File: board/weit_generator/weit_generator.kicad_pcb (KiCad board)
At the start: 2 copper layers, 46 parts, among them J1 POWER, J2 PROG, J3 OUTPUT, U1 MCP6004, U2 AVR32DA28x-xSO, U3 TL431DBZ, X1 SG-5032CCN

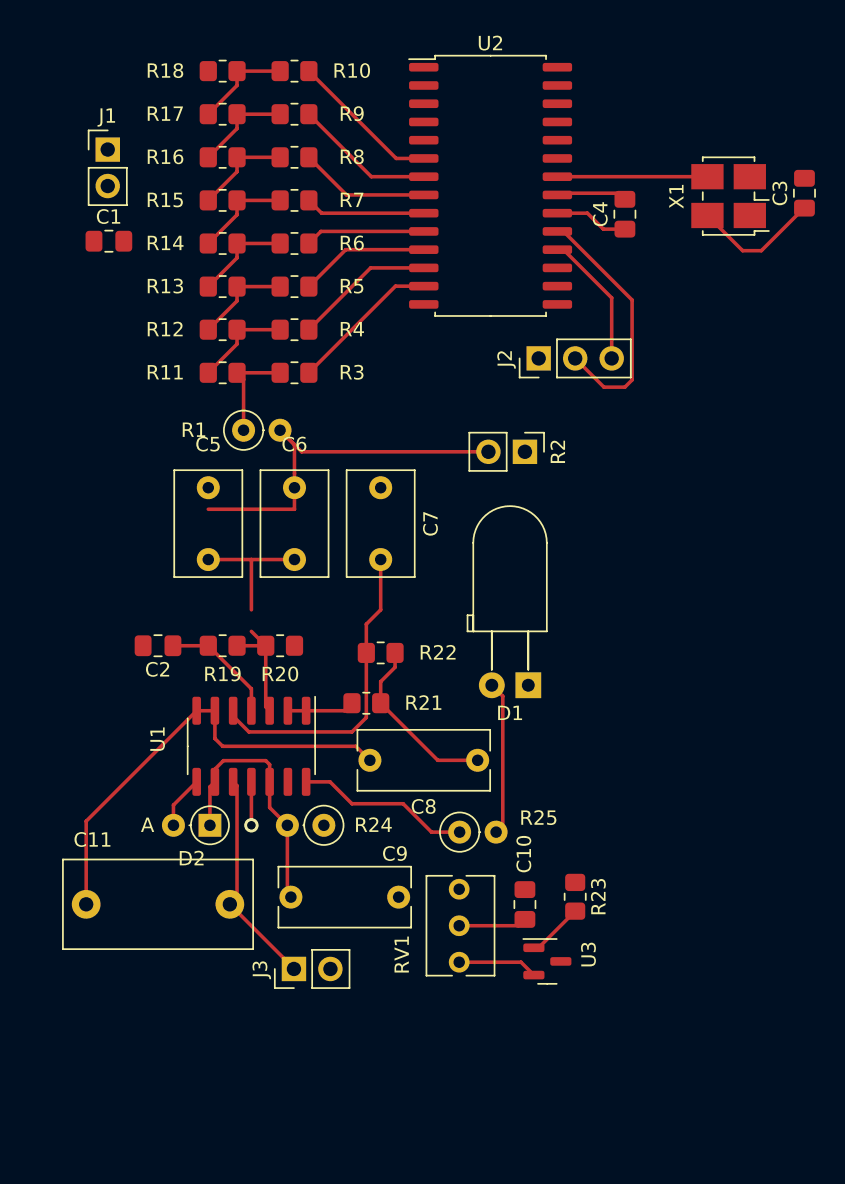
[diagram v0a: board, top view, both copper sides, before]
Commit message: .
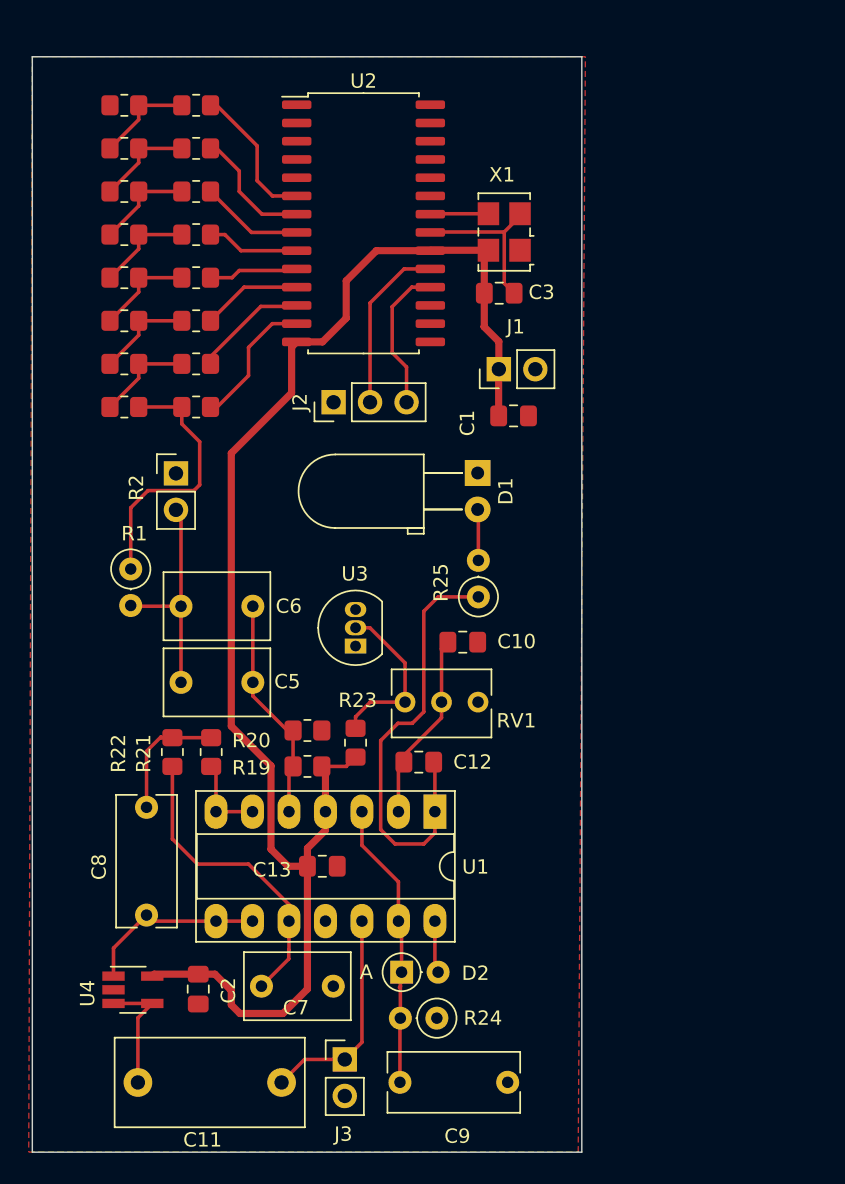
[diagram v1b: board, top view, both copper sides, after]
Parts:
- removed C4: 100n, Capacitor_SMD:C_0805_2012Metric_Pad1.18x1.45mm_HandSolder
- added C12: 1n, Capacitor_SMD:C_0805_2012Metric_Pad1.18x1.45mm_HandSolder, F.Cu at (159.7, 114.1)
- added C13: 100n, Capacitor_SMD:C_0805_2012Metric_Pad1.18x1.45mm_HandSolder, F.Cu at (152.9, 121.3)
- added U4: LMV321, Package_TO_SOT_SMD:SOT-23-5_HandSoldering, F.Cu at (139.8, 129.9)
- R25: value 50 -> 1k
- U1: footprint Package_SO:SOIC-14_3.9x8.7mm_P1.27mm -> Package_DIP:DIP-14_W7.62mm_Socket_LongPads
- U3: value TL431DBZ -> LM4041LP-ADJ; footprint Package_TO_SOT_SMD:SOT-23 -> Package_TO_SOT_THT:TO-92_Inline
- X1: value SG-5032CCN -> SG-5032CAN; footprint Oscillator:Oscillator_SMD_SeikoEpson_SG8002LB-4Pin_5.0x3.2mm_HandSoldering -> Oscillator:Oscillator_SMD_SeikoEpson_SG8002LB-4Pin_5.0x3.2mm
- moved C7 34.9 mm to (153.7, 129.7), turned to 180 degrees
- moved J1 31.2 mm to (165.2, 86.8), turned to 90 degrees
- moved C1 30.7 mm to (166.2, 90.0)
- moved U3 25.7 mm to (155.2, 106.0), turned to 90 degrees
- moved R2 24.3 mm to (142.8, 94.0), turned to 0 degrees
- moved C2 24.1 mm to (144.3, 129.9), turned to -90 degrees
- moved C8 23.3 mm to (140.7, 117.2), turned to -90 degrees
- moved C3 22.4 mm to (165.2, 81.5), turned to 0 degrees
- moved C10 18.8 mm to (162.7, 105.8), turned to 0 degrees
- moved R23 18.7 mm to (155.2, 112.8), turned to 90 degrees
- moved D2 16.8 mm to (158.5, 128.7), turned to 0 degrees
- moved R25 16.4 mm to (163.8, 102.6), turned to 90 degrees
- moved R22 16.1 mm to (142.5, 113.4), turned to -90 degrees
- moved X1 15.8 mm to (165.6, 77.2)
- moved R24 15.6 mm to (160.9, 131.9)
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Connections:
- C10 pad 1: Net-(U1D--) -> Net-(U1A--)
- C11 pad 1: /Output Filter/OUT -> Net-(U4--)
- C5 pad 1: Net-(U1A-+) -> Net-(U1B-+)
- C6 pad 1: Net-(U1A-+) -> Net-(U1B-+)
- C7 pad 2: Net-(U1B-+) -> Net-(U1C-+)
- R19 pad 2: Net-(U1A-+) -> Net-(U1B-+)
- R20 pad 2: Net-(U1A-+) -> Net-(U1B-+)
- R21 pad 1: Net-(U1A--) -> Net-(U1B--)
- R22 pad 2: Net-(U1B-+) -> Net-(U1C-+)
- R25 pad 1: Net-(R25-Pad1) -> Net-(C12-Pad1)
- RV1 pad 2: Net-(U1D--) -> Net-(U1A--)
- U1 pad 1: Net-(U1A--) -> Net-(C12-Pad1)
- U1 pad 10: /OUTPUT -> Net-(U1C-+)
- U1 pad 12: Net-(D2-K) -> /OUTPUT
- U1 pad 13: Net-(U1D--) -> Net-(D2-K)
- U1 pad 14: Net-(R25-Pad1) -> Net-(D2-A)
- U1 pad 3: Net-(U1A-+) -> Net-(D2-K)
- U1 pad 6: /Output Filter/OUT -> Net-(U1B--)
- U1 pad 7: /Output Filter/OUT -> Net-(U1B--)
- U1 pad 8: Net-(D2-A) -> /Output Filter/OUT
- U1 pad 9: Net-(D2-K) -> /Output Filter/OUT
- U3 pad 1: Net-(U3-K) -> unconnected-(U3-FB-Pad1)
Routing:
- net +3V0: track 22.4 -> 103.0 mm
- net Net-(C12-Pad1): track 0.00 -> 30.9 mm
- net Net-(U1C-+): track 0.00 -> 21.5 mm
- net /Output Filter/OUT: track 31.3 -> 12.8 mm
- net Net-(U1A-+): track 17.6 -> 0.00 mm
- net Net-(R25-Pad1): track 12.1 -> 0.00 mm
- net /R-2R DAC/OUT: track 7.19 -> 19.2 mm
- net /Output Filter/IN: track 27.0 -> 15.7 mm
- net Net-(U4--): track 0.00 -> 8.61 mm
- net Net-(U1A--): track 4.68 -> 13.2 mm
- net /Autogain/OUT: track 10.7 -> 3.57 mm
- net Net-(U2-PA0): track 10.4 -> 4.06 mm
- net Net-(U1B-+): track 21.9 -> 15.8 mm
- net Net-(U1B--): track 0.00 -> 5.83 mm
- net Net-(J2-Pin_2): track 17.7 -> 12.1 mm
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- added copper zone on F.Cu, net GND
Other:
- board outline added: 38.2 x 76.2 mm
